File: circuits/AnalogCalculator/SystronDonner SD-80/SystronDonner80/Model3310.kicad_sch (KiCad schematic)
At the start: 0 parts

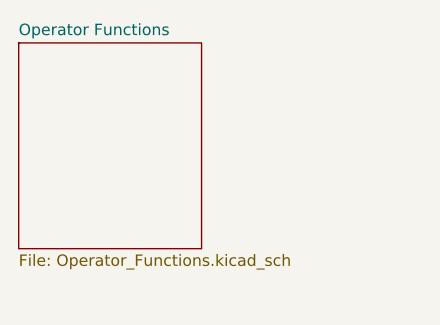
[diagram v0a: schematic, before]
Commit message: update examples
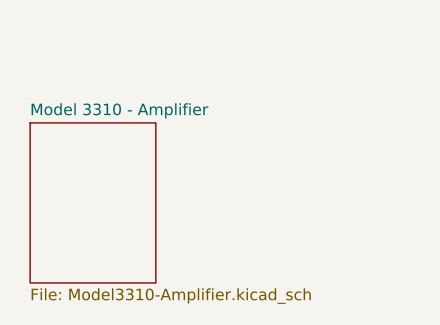
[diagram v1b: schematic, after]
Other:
- removed sheet Operator Functions
- added sheet Model 3310 - Amplifier (Model3310-Amplifier.kicad_sch)
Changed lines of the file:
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@@
 	(paper "A4")
 	(sheet
-		(at 30.48 22.86)
-		(size 20.32 22.86)
+		(at 31.75 31.75)
+		(size 13.97 17.78)
 		(exclude_from_sim no)
 		(in_bom yes)
@@
 			(color 0 0 0 0.0000)
 		)
-		(property "Sheetname" "Operator Functions"
-			(at 30.48 22.1484 0)
+		(property "Sheetname" "Model 3310 - Amplifier"
+			(at 31.75 31.0384 0)
 			(effects
 				(font
@@
 			)
 		)
-		(property "Sheetfile" "Operator_Functions.kicad_sch"
-			(at 30.48 46.3046 0)
+		(property "Sheetfile" "Model3310-Amplifier.kicad_sch"
+			(at 31.75 50.1146 0)
 			(effects
 				(font
@@
 		)
 		(instances
-			(project "ComdynaGp6Clone"
-				(path "/d8186fbb-621b-4e5c-ab25-0b6509cd1564"
-					(page "2")
+			(project "SystronDonner80"
+				(path "/45304ce9-0593-485f-93de-012642aaae97/1b91bcb7-67ef-44b7-be45-d211792f6c4c"
+					(page "3")
 				)
 			)
 		)
 	)
-	(sheet_instances
-		(path "/"
-			(page "1")
-		)
-	)
-	(embedded_fonts no)
 )
